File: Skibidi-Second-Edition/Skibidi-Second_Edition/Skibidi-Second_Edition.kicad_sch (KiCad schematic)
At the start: 69 parts, among them IC1 TEENSY_4.1, J1 Screw_Terminal_01x03, J10 Screw_Terminal_01x03, J12 12V, J13 Conn_01x03_Pin, J14 Conn_01x08_Pin, J15 Conn_02x05_Odd_Even, J16 P78E05-1000, J17 Conn_01x04_Pin, J2 Screw_Terminal_01x03, J3 Screw_Terminal_01x03, J4 Screw_Terminal_01x03, J5 Screw_Terminal_01x03, J6 Screw_Terminal_01x03, J7 Screw_Terminal_01x03, J8 Screw_Terminal_01x03, SW1 SW_Nidec_CAS-120A1, SW2 210-4MS

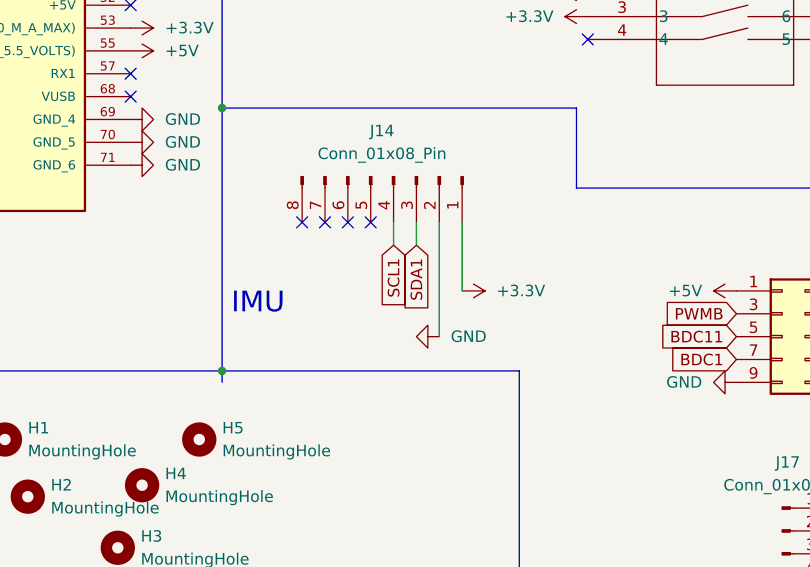
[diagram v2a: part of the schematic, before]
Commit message: wf
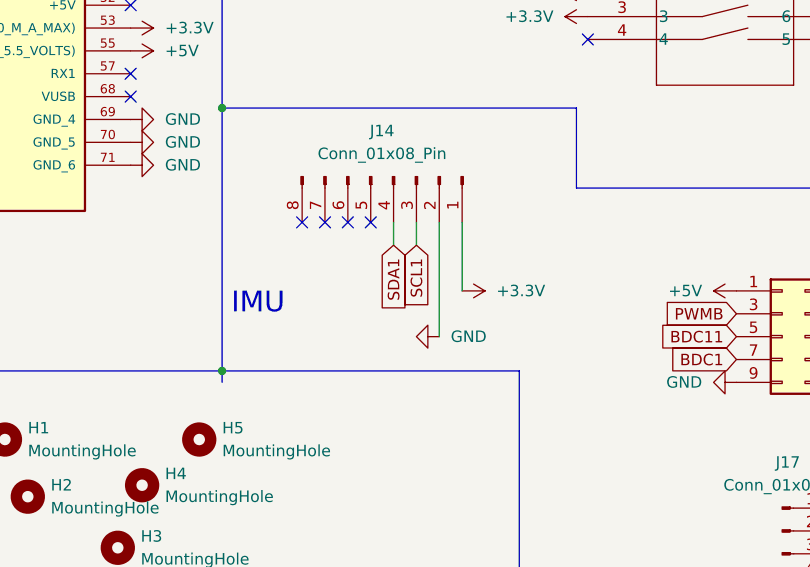
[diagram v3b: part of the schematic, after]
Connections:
- net SCL1: now also J14.3 (Pin_3); no longer J14.4 (Pin_4)
- net SDA1: now also J14.4 (Pin_4); no longer J14.3 (Pin_3)
